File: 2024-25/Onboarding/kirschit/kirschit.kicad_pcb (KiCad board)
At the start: 2 copper layers, 56.5 x 42.5 mm, 6 parts, among them J1 Conn_01x04, J2 Conn_01x02, SW1 SW_SPST, SW2 SW_SPST

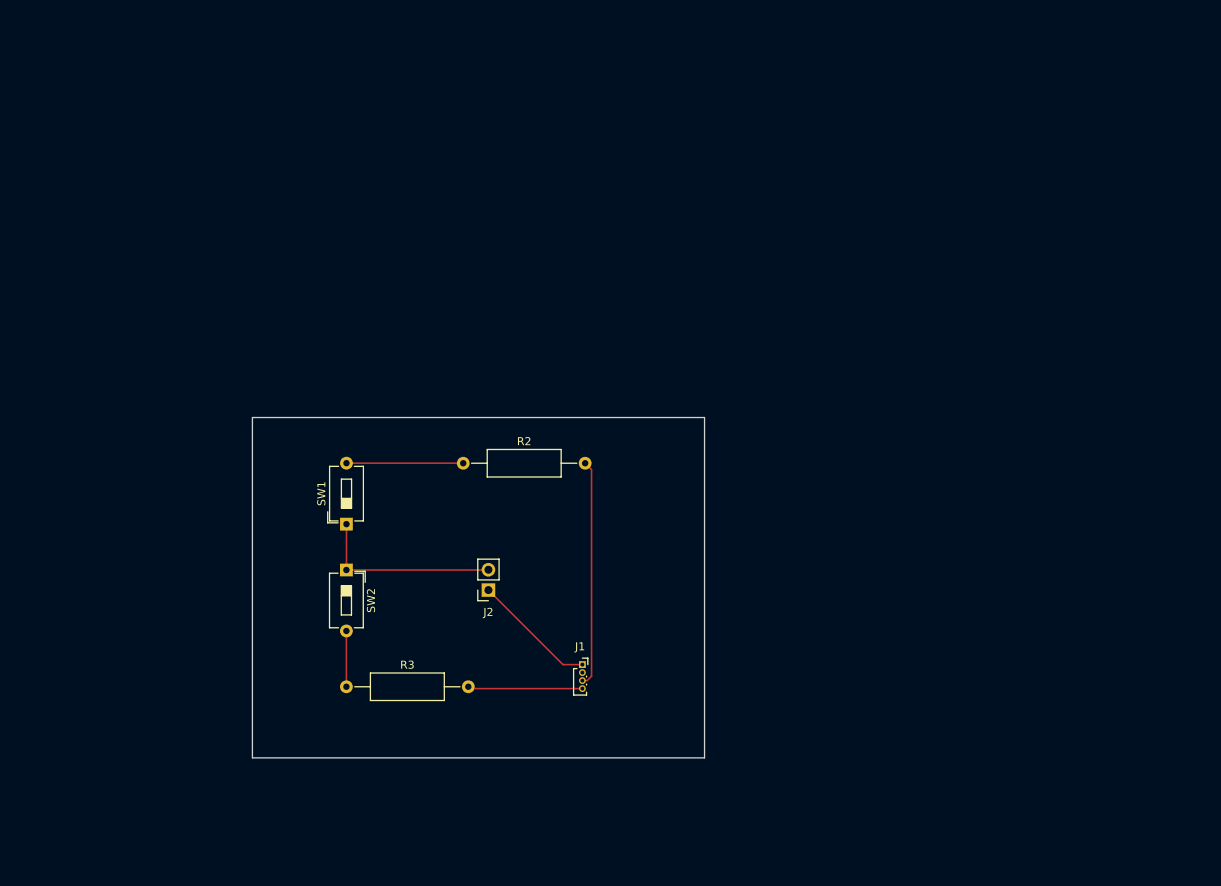
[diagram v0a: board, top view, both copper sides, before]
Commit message: Finished schematic
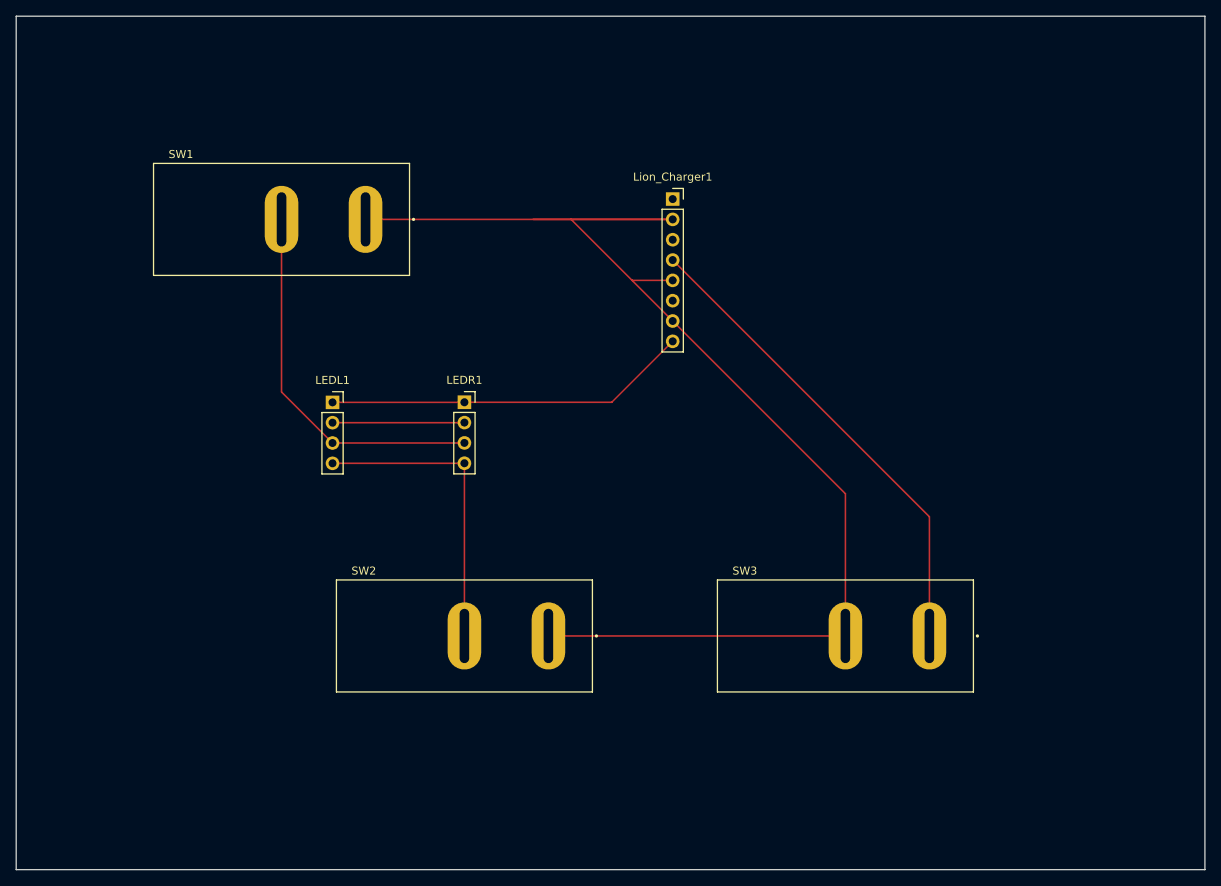
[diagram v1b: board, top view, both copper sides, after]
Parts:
- removed J1: Conn_01x04, Connector_PinSocket_1.00mm:PinSocket_1x04_P1.00mm_Vertical
- removed J2: Conn_01x02, Connector_PinSocket_2.54mm:PinSocket_1x02_P2.54mm_Vertical
- removed R2, R3: 330, Resistor_THT:R_Axial_DIN0309_L9.0mm_D3.2mm_P15.24mm_Horizontal
- added LEDL1: Conn_01x04, Connector_PinSocket_2.54mm:PinSocket_1x04_P2.54mm_Vertical, F.Cu at (110.7, 88.3)
- added LEDR1: Conn_01x04, Connector_PinSocket_2.54mm:PinSocket_1x04_P2.54mm_Vertical, F.Cu at (127.1, 88.3)
- added Lion_Charger1: Conn_01x08, Connector_PinSocket_2.54mm:PinSocket_1x08_P2.54mm_Vertical, F.Cu at (153.2, 62.9)
- added SW3: EN, RB141C1100:SW_RB141C1100, F.Cu at (174.8, 117.5)
- SW1: value SW_SPST -> LEDR; footprint Button_Switch_THT:SW_DIP_SPSTx01_Slide_6.7x4.1mm_W7.62mm_P2.54mm_LowProfile -> RB141C1100:SW_RB141C1100
- SW2: value SW_SPST -> LEDB; footprint Button_Switch_THT:SW_DIP_SPSTx01_Slide_6.7x4.1mm_W7.62mm_P2.54mm_LowProfile -> RB141C1100:SW_RB141C1100
- moved SW1 38.9 mm to (104.3, 65.4), turned to 0 degrees
- moved SW2 16.9 mm to (127.1, 117.5), turned to 0 degrees
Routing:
- net /GND: track 23.5 -> 164.3 mm
- net /EN: track 0.00 -> 60.3 mm
- net /LEDR: track 14.6 -> 47.7 mm
- net /LEDB: track 6.98 -> 38.1 mm
- net /5V: track 15.6 -> 45.7 mm
- net Net-(J1-Pin_3): track 28.3 -> 0.00 mm
- net /LEDG: track 0.00 -> 16.5 mm
- net Net-(J1-Pin_4): track 14.4 -> 0.00 mm
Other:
- board size 56.5 x 42.5 mm -> 148.6 x 106.7 mm
